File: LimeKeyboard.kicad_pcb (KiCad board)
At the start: 2 copper layers, 134.6 x 109.9 mm, 103 parts, among them J2 4PIN, J3 OLED, P1 i2c_pin, P2 i2c_pin, SW1 SW_PUSH, SW10 SW_PUSH, SW11 SW_PUSH, SW12 SW_PUSH, SW13 SW_PUSH, SW14 SW_PUSH, SW15 SW_PUSH, SW16 SW_PUSH, SW17 SW_PUSH, SW18 SW_PUSH, SW19 SW_PUSH, SW2 SW_PUSH, SW20 SW_PUSH, SW21 SW_PUSH, SW22 SW_PUSH, SW23 SW_PUSH, SW24 SW_PUSH, SW25 SW_PUSH, SW26 SW_PUSH, SW27 SW_PUSH, SW28 SW_PUSH, SW29 SW_PUSH, SW3 SW_PUSH, SW30 SW_PUSH, SW31 Rotary_Encoder_Switch, SW4 SW_PUSH, SW5 SW_PUSH, SW6 SW_PUSH, SW7 SW_PUSH, SW8 SW_PUSH, SW9 SW_PUSH, U1 ProMicro

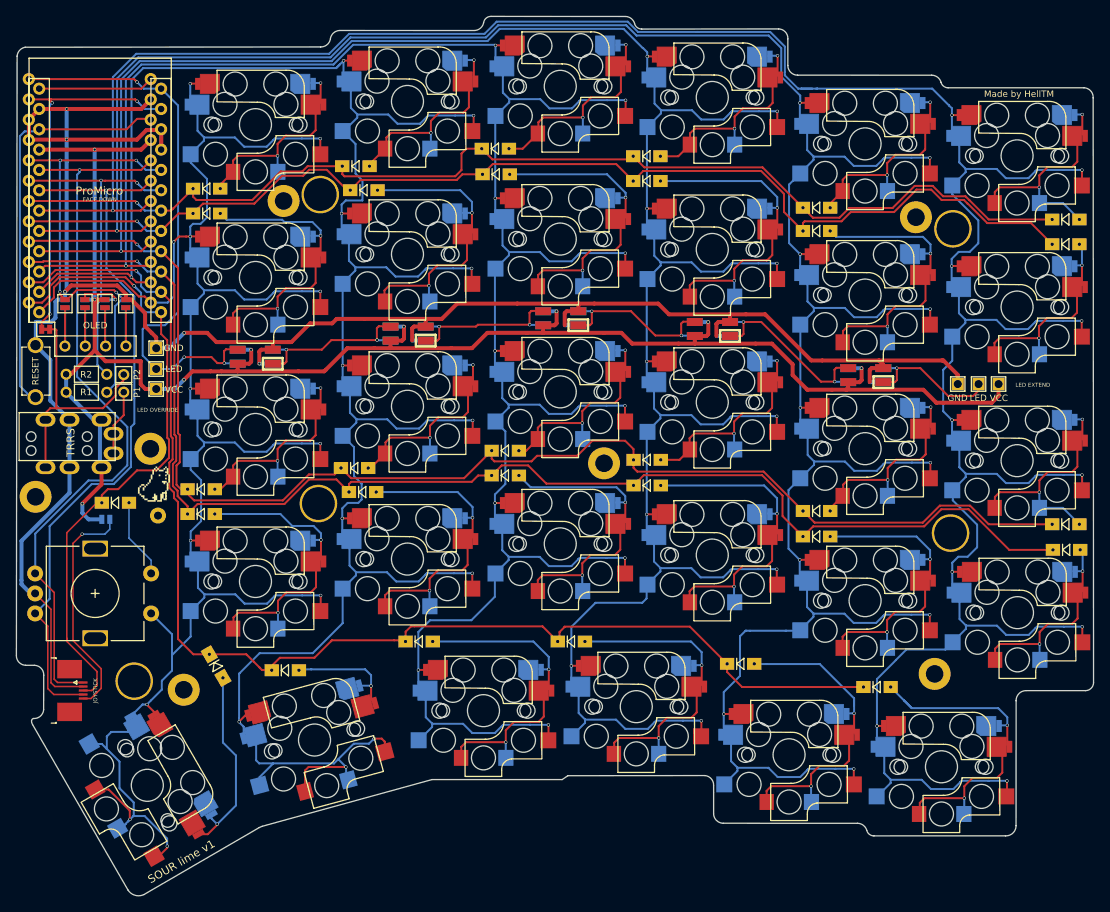
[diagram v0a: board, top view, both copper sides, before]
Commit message: made sure things are all local to this project
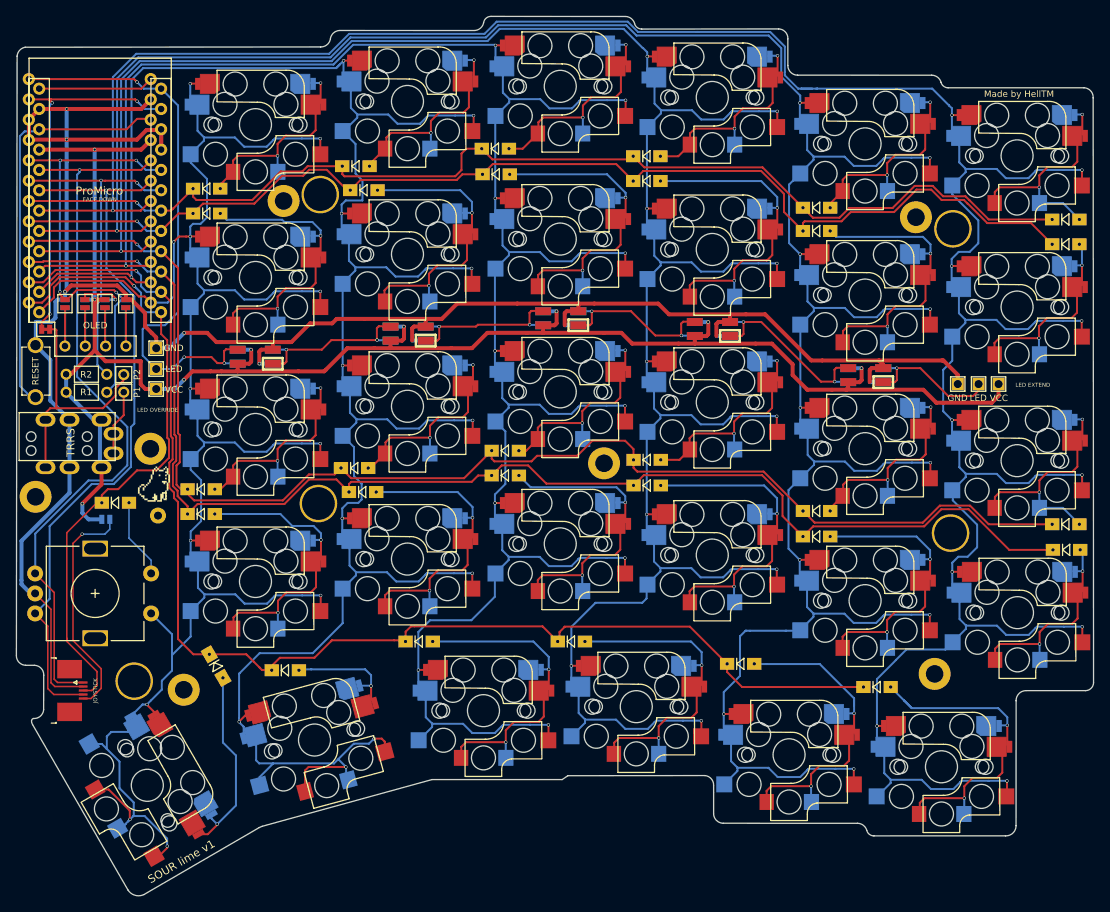
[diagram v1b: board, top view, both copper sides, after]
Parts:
- JP6: value Jumper_Joystick -> Jumper_NO_Small
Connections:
- D1 pad 1: (no net) -> row0
- D1 pad 2: (no net) -> Net-(D1-Pad2)
- D10 pad 1: (no net) -> row1
- D10 pad 2: (no net) -> Net-(D10-Pad2)
- D11 pad 1: (no net) -> row1
- D11 pad 2: (no net) -> Net-(D11-Pad2)
- D12 pad 1: (no net) -> row1
- D12 pad 2: (no net) -> Net-(D12-Pad2)
- D13 pad 1: (no net) -> row2
- D13 pad 2: (no net) -> Net-(D13-Pad2)
- D14 pad 1: (no net) -> row2
- D14 pad 2: (no net) -> Net-(D14-Pad2)
- D15 pad 1: (no net) -> row2
- D15 pad 2: (no net) -> Net-(D15-Pad2)
- D16 pad 1: (no net) -> row2
- D16 pad 2: (no net) -> Net-(D16-Pad2)
- D17 pad 1: (no net) -> row2
- D17 pad 2: (no net) -> Net-(D17-Pad2)
- D18 pad 1: (no net) -> row2
- D18 pad 2: (no net) -> Net-(D18-Pad2)
- D19 pad 1: (no net) -> row3
- D19 pad 2: (no net) -> Net-(D19-Pad2)
- D2 pad 1: (no net) -> row0
- D2 pad 2: (no net) -> Net-(D2-Pad2)
- D20 pad 1: (no net) -> row3
- D20 pad 2: (no net) -> Net-(D20-Pad2)
- D21 pad 1: (no net) -> row3
- D21 pad 2: (no net) -> Net-(D21-Pad2)
- D22 pad 1: (no net) -> row3
- D22 pad 2: (no net) -> Net-(D22-Pad2)
- D23 pad 1: (no net) -> row3
- D23 pad 2: (no net) -> Net-(D23-Pad2)
- D24 pad 1: (no net) -> row3
- D24 pad 2: (no net) -> Net-(D24-Pad2)
- D25 pad 1: (no net) -> row4
- D25 pad 2: (no net) -> Net-(D25-Pad2)
- D26 pad 1: (no net) -> row4
- D26 pad 2: (no net) -> Net-(D26-Pad2)
- D27 pad 1: (no net) -> row4
- D27 pad 2: (no net) -> Net-(D27-Pad2)
- D28 pad 1: (no net) -> row4
- D28 pad 2: (no net) -> Net-(D28-Pad2)
- D29 pad 1: (no net) -> row4
- D29 pad 2: (no net) -> Net-(D29-Pad2)
- D3 pad 1: (no net) -> row0
- D3 pad 2: (no net) -> Net-(D3-Pad2)
- D30 pad 1: (no net) -> row4
- D30 pad 2: (no net) -> Net-(D30-Pad2)
- D31 pad 1: (no net) -> row5
- D31 pad 2: (no net) -> SW31B
- D4 pad 1: (no net) -> row0
- D4 pad 2: (no net) -> Net-(D4-Pad2)
- D5 pad 1: (no net) -> row0
- D5 pad 2: (no net) -> Net-(D5-Pad2)
- D6 pad 1: (no net) -> row0
- D6 pad 2: (no net) -> Net-(D6-Pad2)
- D7 pad 1: (no net) -> row1
- D7 pad 2: (no net) -> Net-(D7-Pad2)
- D8 pad 1: (no net) -> row1
- D8 pad 2: (no net) -> Net-(D8-Pad2)
- D9 pad 1: (no net) -> row1
- D9 pad 2: (no net) -> Net-(D9-Pad2)
- J2 pad 1: (no net) -> VCC
- J2 pad 2: (no net) -> GND
- J2 pad 3: (no net) -> /i2c_d
- J2 pad 4: (no net) -> /i2c_c
- J3 pad 1: (no net) -> Net-(J3-Pad1)
- J3 pad 2: (no net) -> Net-(J3-Pad2)
- J3 pad 3: (no net) -> Net-(J3-Pad3)
- J3 pad 4: (no net) -> Net-(J3-Pad4)
- JP1 pad 1: (no net) -> Net-(J3-Pad4)
- JP1 pad 2: (no net) -> GND
- JP2 pad 1: (no net) -> Net-(J3-Pad3)
- JP2 pad 2: (no net) -> VCC
- JP3 pad 1: (no net) -> Net-(J3-Pad2)
- JP3 pad 2: (no net) -> SCL
- JP4 pad 1: (no net) -> Net-(J3-Pad1)
- JP4 pad 2: (no net) -> SDA
- JP5 pad 1: (no net) -> Net-(J3-Pad4)
- JP5 pad 2: (no net) -> SDA
- JP6 pad 1: (no net) -> Net-(J3-Pad3) (x2)
- JP6 pad 2: (no net) -> SCL (x2)
- JP7 pad 1: (no net) -> Net-(J3-Pad2)
- JP7 pad 2: (no net) -> VCC
- JP8 pad 1: (no net) -> Net-(J3-Pad1)
- JP8 pad 2: (no net) -> GND
- P1 pad 1: (no net) -> /i2c_c
- P2 pad 1: (no net) -> /i2c_d
- R1 pad 1: (no net) -> VCC
- R1 pad 2: (no net) -> SDA
- R2 pad 1: (no net) -> VCC
- R2 pad 2: (no net) -> SCL
- RSW1 pad 1: (no net) -> GND
- RSW1 pad 2: (no net) -> RESET
- SW1 pad 1: (no net) -> SW31A
- SW1 pad 2: (no net) -> Net-(D1-Pad2)
- SW10 pad 1: (no net) -> col2
- SW10 pad 2: (no net) -> Net-(D10-Pad2)
- SW11 pad 1: (no net) -> col1
- SW11 pad 2: (no net) -> Net-(D11-Pad2)
- SW12 pad 1: (no net) -> col0
- SW12 pad 2: (no net) -> Net-(D12-Pad2)
- SW13 pad 1: (no net) -> SW31A
- SW13 pad 2: (no net) -> Net-(D13-Pad2)
- SW14 pad 1: (no net) -> col4
- SW14 pad 2: (no net) -> Net-(D14-Pad2)
- SW15 pad 1: (no net) -> col3
- SW15 pad 2: (no net) -> Net-(D15-Pad2)
- SW16 pad 1: (no net) -> col2
- SW16 pad 2: (no net) -> Net-(D16-Pad2)
- SW17 pad 1: (no net) -> col1
- SW17 pad 2: (no net) -> Net-(D17-Pad2)
- SW18 pad 1: (no net) -> col0
- SW18 pad 2: (no net) -> Net-(D18-Pad2)
- SW19 pad 1: (no net) -> SW31A
- SW19 pad 2: (no net) -> Net-(D19-Pad2)
- SW2 pad 1: (no net) -> col4
- SW2 pad 2: (no net) -> Net-(D2-Pad2)
- SW20 pad 1: (no net) -> col4
- SW20 pad 2: (no net) -> Net-(D20-Pad2)
- SW21 pad 1: (no net) -> col3
- SW21 pad 2: (no net) -> Net-(D21-Pad2)
- SW22 pad 1: (no net) -> col2
- SW22 pad 2: (no net) -> Net-(D22-Pad2)
- SW23 pad 1: (no net) -> col1
- SW23 pad 2: (no net) -> Net-(D23-Pad2)
- SW24 pad 1: (no net) -> col0
- SW24 pad 2: (no net) -> Net-(D24-Pad2)
- SW25 pad 1: (no net) -> SW31A
- SW25 pad 2: (no net) -> Net-(D25-Pad2)
- SW26 pad 1: (no net) -> col4
- SW26 pad 2: (no net) -> Net-(D26-Pad2)
- SW27 pad 1: (no net) -> col3
- SW27 pad 2: (no net) -> Net-(D27-Pad2)
- SW28 pad 1: (no net) -> col2
- SW28 pad 2: (no net) -> Net-(D28-Pad2)
- SW29 pad 1: (no net) -> col1
- SW29 pad 2: (no net) -> Net-(D29-Pad2)
- SW3 pad 1: (no net) -> col3
- SW3 pad 2: (no net) -> Net-(D3-Pad2)
- SW30 pad 1: (no net) -> col0
- SW30 pad 2: (no net) -> Net-(D30-Pad2)
- SW31 pad A: (no net) -> ENCA
- SW31 pad B: (no net) -> ENCB
- SW31 pad C: (no net) -> GND
- SW31 pad S1: (no net) -> SW31A
- SW31 pad S2: (no net) -> SW31B
- SW4 pad 1: (no net) -> col2
- SW4 pad 2: (no net) -> Net-(D4-Pad2)
- SW5 pad 1: (no net) -> col1
- SW5 pad 2: (no net) -> Net-(D5-Pad2)
- SW6 pad 1: (no net) -> col0
- SW6 pad 2: (no net) -> Net-(D6-Pad2)
- SW7 pad 1: (no net) -> SW31A
- SW7 pad 2: (no net) -> Net-(D7-Pad2)
- SW8 pad 1: (no net) -> col4
- SW8 pad 2: (no net) -> Net-(D8-Pad2)
- SW9 pad 1: (no net) -> col3
- SW9 pad 2: (no net) -> Net-(D9-Pad2)
- U1 pad 1: (no net) -> LED
- U1 pad 10: (no net) -> row3
- U1 pad 11: (no net) -> row4
- U1 pad 12: (no net) -> row5
- U1 pad 13: (no net) -> SW31A
- U1 pad 14: (no net) -> col4
- U1 pad 15: (no net) -> col3
- U1 pad 16: (no net) -> col2
- U1 pad 17: (no net) -> col1
- U1 pad 18: (no net) -> col0
- U1 pad 19: (no net) -> ENCB
- U1 pad 2: (no net) -> DATA
- U1 pad 20: (no net) -> ENCA
- U1 pad 21: (no net) -> VCC
- U1 pad 22: (no net) -> RESET
- U1 pad 23: (no net) -> GND
- U1 pad 24: (no net) -> unconnected-(U1-Pad24)
- U1 pad 3: (no net) -> GND
- U1 pad 4: (no net) -> GND
- U1 pad 5: (no net) -> SDA
- U1 pad 6: (no net) -> SCL
- U1 pad 7: (no net) -> row0
- U1 pad 8: (no net) -> row1
- U1 pad 9: (no net) -> row2
- W1 pad 1: (no net) -> DATA
- W1 pad 2: (no net) -> /i2c_d
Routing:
- net (no net): track 4798.8 -> 114.5 mm, vias 171 -> 9
- net col0: track 0.00 -> 349.2 mm, vias 0 -> 11
- net col1: track 0.00 -> 321.4 mm, vias 0 -> 11
- net col2: track 0.00 -> 297.9 mm, vias 0 -> 11
- net col4: track 0.00 -> 286.4 mm, vias 0 -> 12
- net col3: track 0.00 -> 279.6 mm, vias 0 -> 11
- net GND: track 0.00 -> 275.8 mm, vias 0 -> 5
- net SW31A: track 0.00 -> 241.7 mm, vias 0 -> 12
- net VCC: track 0.00 -> 228.0 mm, vias 0 -> 9
- net row2: track 0.00 -> 172.1 mm, vias 0 -> 1
- net row3: track 0.00 -> 171.5 mm, vias 0 -> 1
- net row4: track 0.00 -> 161.1 mm, vias 0 -> 1
- net row1: track 0.00 -> 146.1 mm, vias 0 -> 1
- net row0: track 0.00 -> 143.5 mm, vias 0 -> 1
- net ENCA: track 0.00 -> 92.1 mm, vias 0 -> 1
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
